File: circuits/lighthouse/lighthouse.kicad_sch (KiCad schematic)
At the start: 45 parts, among them J1 USB_C_Receptacle_USB2.0_14P, J2 Conn_01x03_Socket, Q1 S9013, Q4 SS8050, Q5 SS8050, U10 CP2102-GMR, U2 AMS1117-3.3, U7 ESP32-WROOM-32

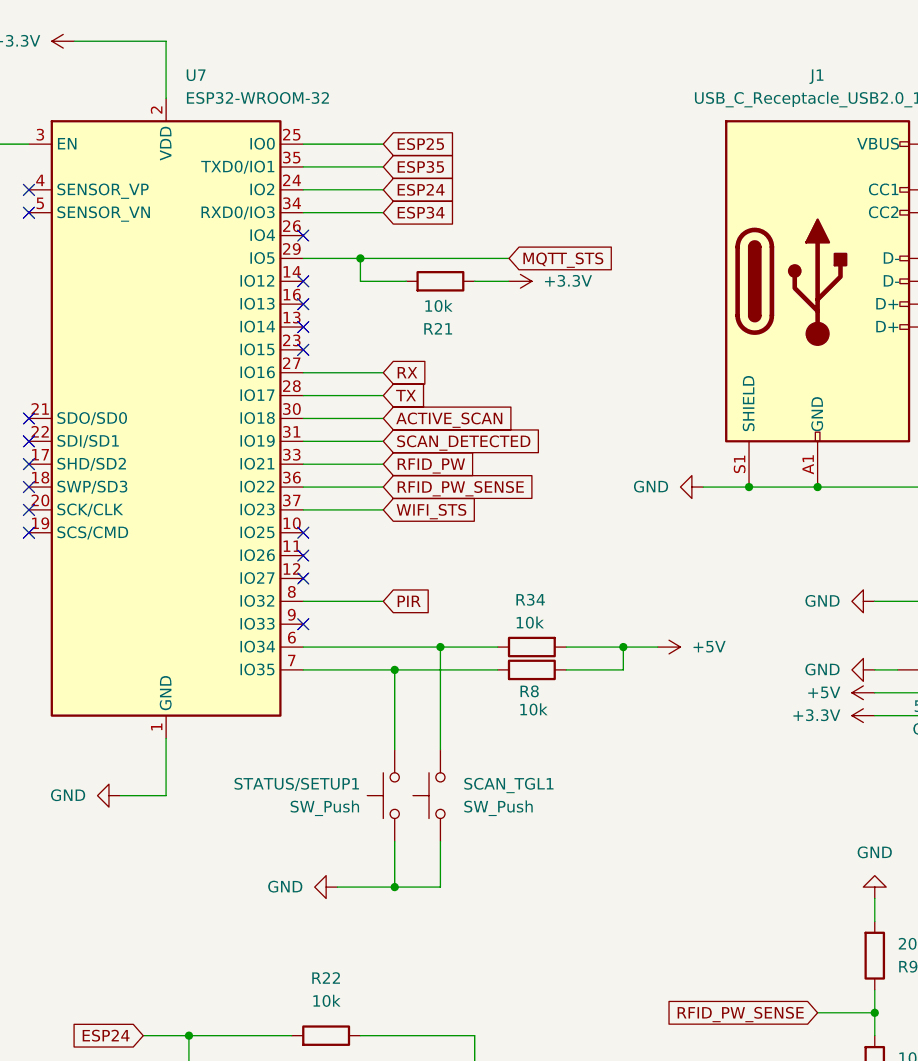
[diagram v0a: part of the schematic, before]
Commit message: Ready to go circuit (what a naive thing to say)
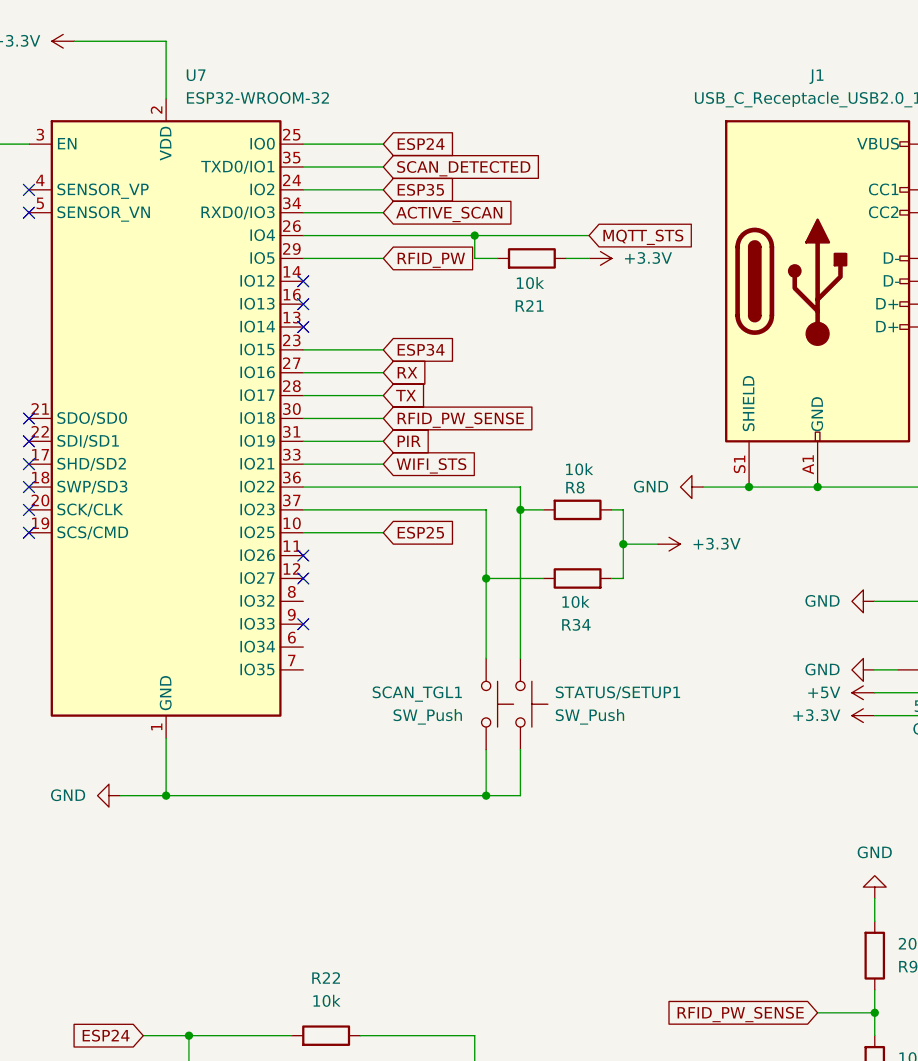
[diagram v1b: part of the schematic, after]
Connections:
- net +3.3V: now also R34.2, R8.1
- net +5V: no longer R34.2, R8.1
- net ACTIVE_SCAN: now also U7.34 (RXD0/IO3); no longer U7.30 (IO18)
- net ESP24: now also U7.25 (IO0); no longer U7.24 (IO2)
- net ESP25: now also U7.10 (IO25); no longer U7.25 (IO0)
- net ESP34: now also U7.23 (IO15); no longer U7.34 (RXD0/IO3)
- net ESP35: now also U7.24 (IO2); no longer U7.35 (TXD0/IO1)
- net MQTT_STS: now also U7.26 (IO4); no longer U7.29 (IO5)
- net PIR: now also U7.31 (IO19); no longer U7.8 (IO32)
- net RFID_PW: now also U7.29 (IO5); no longer U7.33 (IO21)
- net RFID_PW_SENSE: now also U7.30 (IO18); no longer U7.36 (IO22)
- net SCAN_DETECTED: now also U7.35 (TXD0/IO1); no longer U7.31 (IO19)
- net WIFI_STS: now also U7.33 (IO21); no longer U7.37 (IO23)
- net at R34.1, SCAN_TGL1.2: now also U7.37 (IO23); no longer U7.6 (IO34)
- net at R8.2, STATUS/SETUP1.2: now also U7.36 (IO22); no longer U7.7 (IO35)
- no-connect marks 25 -> 22
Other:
- moved on the sheet: R21, R34, R8, SCAN_TGL1, STATUS/SETUP1
